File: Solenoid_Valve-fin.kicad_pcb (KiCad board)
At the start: 2 copper layers, 85.9 x 100 mm, 118 parts, among them IC1 Si8621AB-B-ISR, J1 Bus_mechaken_PCIexpress_x16_1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, J10 Conn_01x02, J11 Conn_01x02, J12 Conn_01x02, J13 Conn_01x02, J14 Conn_01x02, J15 Conn_01x02, J16 Conn_01x02, J17 Conn_01x02, J18 Conn_01x02, J19 Conn_01x02, J2 Conn_01x05, J20 Conn_01x02, J3 Conn_01x02, J4 Conn_01x02, J5 Conn_01x02, J6 Conn_01x02, J7 Conn_01x03, J8 Conn_01x02, J9 Conn_01x02, Q1 ULN2004D1013TR, Q2 ULN2004D1013TR, Q3 ULN2004D1013TR, U1 LDL1117S33R, U2 STM32F042K6Tx, U3 MCP2562-E-SN, U4 L7812, U5 LDL1117S33R

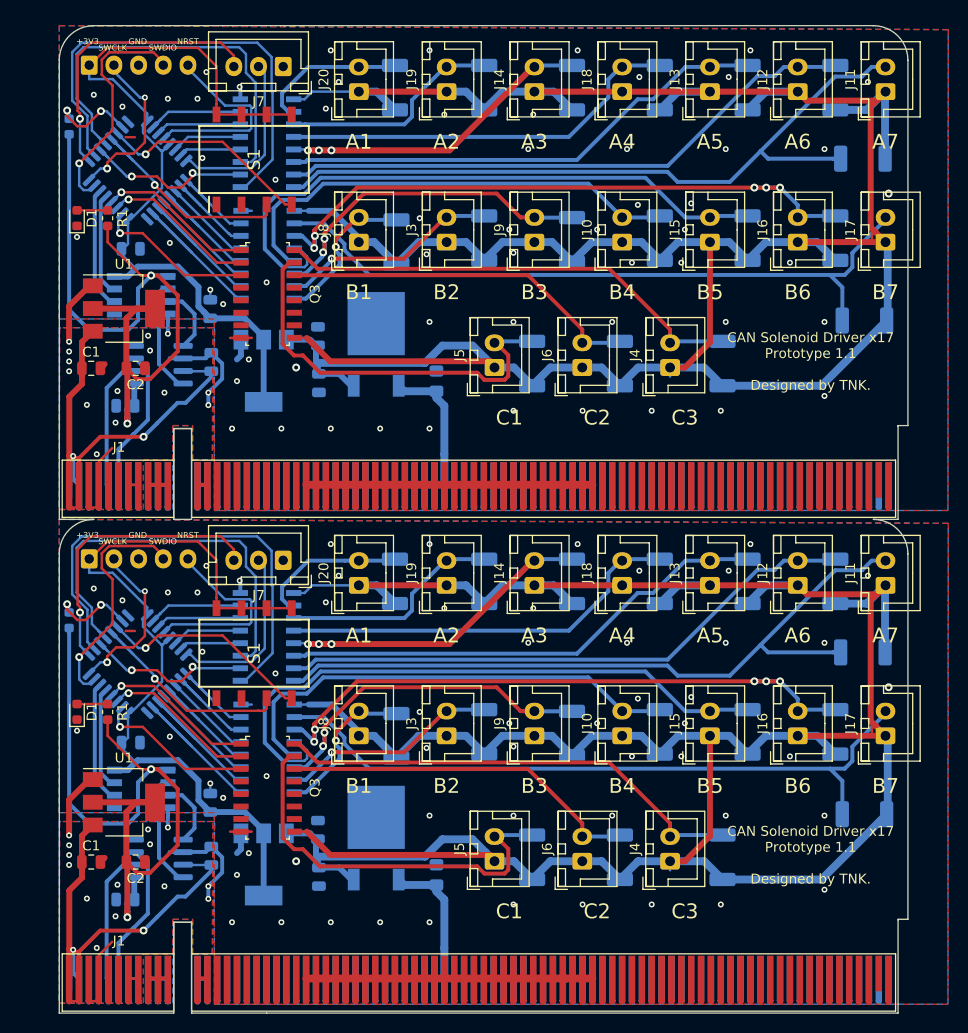
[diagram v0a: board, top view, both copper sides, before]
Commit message: Release
Prototype-1.3をリリース
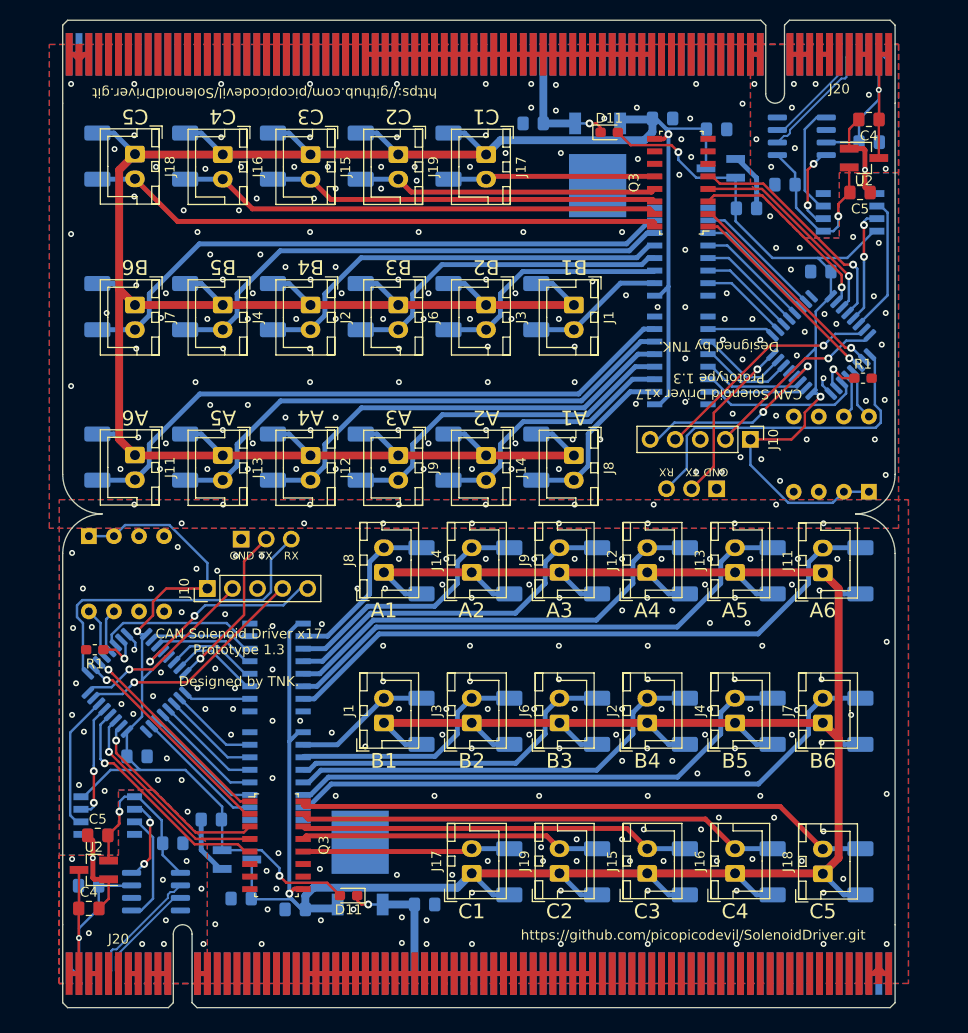
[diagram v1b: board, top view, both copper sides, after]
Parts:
- removed C10: 4.7uF, Capacitor_SMD:C_0805_2012Metric
- removed the D1 at (121.8, 49.5)
- removed the D1 at (121.8, 99.5)
- removed the D11 at (198.6, 36.3)
- removed D19: D, Diode_SMD:D_2010_5025Metric
- removed the R1 at (124.9, 49.5)
- removed the R1 at (124.9, 99.5)
- removed R2: 10K, Resistor_SMD:R_0603_1608Metric
- added C3: 0.1u, Capacitor_SMD:C_0805_2012Metric_Pad1.15x1.40mm_HandSolder, B.Cu at (181.1, 39.4)
- added D1: D, Diode_SMD:D_2010_5025Metric_Pad1.52x2.65mm_HandSolder, B.Cu at (168.3, 58.5)
- added D11: D_Schottky, Diode_SMD:D_0603_1608Metric_Pad1.05x0.95mm_HandSolder, F.Cu at (175.7, 40.8)
- added D11: D_Schottky, Diode_SMD:D_0603_1608Metric_Pad1.05x0.95mm_HandSolder, F.Cu at (149.3, 118.1)
- added D5: D, Diode_SMD:D_2010_5025Metric_Pad1.52x2.65mm_HandSolder, B.Cu at (150.5, 58.5)
- added R1: 10K, Resistor_SMD:R_0603_1608Metric_Pad1.05x0.95mm_HandSolder, F.Cu at (201.4, 65.7)
- C1: value 1.0uF -> 0.1u; footprint Capacitor_SMD:C_0805_2012Metric -> Capacitor_SMD:C_0805_2012Metric_Pad1.15x1.40mm_HandSolder; moved to B.Cu
- C1: renamed from C4; value 0.1uF -> 0.1u; footprint Capacitor_SMD:C_0805_2012Metric -> Capacitor_SMD:C_0805_2012Metric_Pad1.15x1.40mm_HandSolder
- C2: value 4.7uF -> 0.33u; footprint Capacitor_SMD:C_0805_2012Metric -> Capacitor_SMD:C_0805_2012Metric_Pad1.15x1.40mm_HandSolder; moved to B.Cu
- C2: renamed from C7; value 1uF -> 0.33u
- C3: renamed from C8; value 4.7uF -> 0.1u; footprint Capacitor_SMD:C_0805_2012Metric -> Capacitor_SMD:C_0805_2012Metric_Pad1.15x1.40mm_HandSolder
- C4: value 0.1uF -> 1.0u; footprint Capacitor_SMD:C_0805_2012Metric -> Capacitor_SMD:C_0805_2012Metric_Pad1.15x1.40mm_HandSolder; moved to F.Cu
- C4: renamed from C1; value 1.0uF -> 1.0u; footprint Capacitor_SMD:C_0805_2012Metric -> Capacitor_SMD:C_0805_2012Metric_Pad1.15x1.40mm_HandSolder
- C5: value 0.1uF -> 2.2u; footprint Capacitor_SMD:C_0805_2012Metric -> Capacitor_SMD:C_0805_2012Metric_Pad1.15x1.40mm_HandSolder; moved to F.Cu
- C5: renamed from C2; value 4.7uF -> 2.2u; footprint Capacitor_SMD:C_0805_2012Metric -> Capacitor_SMD:C_0805_2012Metric_Pad1.15x1.40mm_HandSolder
- C6 (x2): value 0.1uF -> 0.1u; footprint Capacitor_SMD:C_0805_2012Metric -> Capacitor_SMD:C_0805_2012Metric_Pad1.15x1.40mm_HandSolder
- C7: value 1uF -> 1.0u
- C7: renamed from C9; value 1.0uF -> 1.0u; footprint Capacitor_SMD:C_0805_2012Metric -> Capacitor_SMD:C_0805_2012Metric_Pad1.15x1.40mm_HandSolder
- C8: value 4.7uF -> 4.7u; footprint Capacitor_SMD:C_0805_2012Metric -> Capacitor_SMD:C_0805_2012Metric_Pad1.15x1.40mm_HandSolder
- C8: renamed from C10; value 4.7uF -> 4.7u; footprint Capacitor_SMD:C_0805_2012Metric -> Capacitor_SMD:C_0805_2012Metric_Pad1.15x1.40mm_HandSolder
- C9: value 1.0uF -> 0.1u; footprint Capacitor_SMD:C_0805_2012Metric -> Capacitor_SMD:C_0805_2012Metric_Pad1.15x1.40mm_HandSolder
- C9: renamed from C5; value 0.1uF -> 0.1u; footprint Capacitor_SMD:C_0805_2012Metric -> Capacitor_SMD:C_0805_2012Metric_Pad1.15x1.40mm_HandSolder
- D1: renamed from D6; footprint Diode_SMD:D_2010_5025Metric -> Diode_SMD:D_2010_5025Metric_Pad1.52x2.65mm_HandSolder
- D10, D12 (x2), D13, D14, D15, D16, D17, D18, D2, D3, D4, D6, D7, D8, D9: footprint Diode_SMD:D_2010_5025Metric -> Diode_SMD:D_2010_5025Metric_Pad1.52x2.65mm_HandSolder
- D10: renamed from D17; footprint Diode_SMD:D_2010_5025Metric -> Diode_SMD:D_2010_5025Metric_Pad1.52x2.65mm_HandSolder
- D13: renamed from D18; footprint Diode_SMD:D_2010_5025Metric -> Diode_SMD:D_2010_5025Metric_Pad1.52x2.65mm_HandSolder
- D14: renamed from D2; footprint Diode_SMD:D_2010_5025Metric -> Diode_SMD:D_2010_5025Metric_Pad1.52x2.65mm_HandSolder
- D15: renamed from D16; footprint Diode_SMD:D_2010_5025Metric -> Diode_SMD:D_2010_5025Metric_Pad1.52x2.65mm_HandSolder
- D16: renamed from D3; footprint Diode_SMD:D_2010_5025Metric -> Diode_SMD:D_2010_5025Metric_Pad1.52x2.65mm_HandSolder
- D17: renamed from D10; footprint Diode_SMD:D_2010_5025Metric -> Diode_SMD:D_2010_5025Metric_Pad1.52x2.65mm_HandSolder
- D18: renamed from D4; footprint Diode_SMD:D_2010_5025Metric -> Diode_SMD:D_2010_5025Metric_Pad1.52x2.65mm_HandSolder
- D2: renamed from D9; footprint Diode_SMD:D_2010_5025Metric -> Diode_SMD:D_2010_5025Metric_Pad1.52x2.65mm_HandSolder
- D3: renamed from D7; footprint Diode_SMD:D_2010_5025Metric -> Diode_SMD:D_2010_5025Metric_Pad1.52x2.65mm_HandSolder
- D4: renamed from D14; footprint Diode_SMD:D_2010_5025Metric -> Diode_SMD:D_2010_5025Metric_Pad1.52x2.65mm_HandSolder
- D5: renamed from D8; footprint Diode_SMD:D_2010_5025Metric -> Diode_SMD:D_2010_5025Metric_Pad1.52x2.65mm_HandSolder
- D6: renamed from D15; footprint Diode_SMD:D_2010_5025Metric -> Diode_SMD:D_2010_5025Metric_Pad1.52x2.65mm_HandSolder
- D7: renamed from D19; footprint Diode_SMD:D_2010_5025Metric -> Diode_SMD:D_2010_5025Metric_Pad1.52x2.65mm_HandSolder
- D8: renamed from D13; footprint Diode_SMD:D_2010_5025Metric -> Diode_SMD:D_2010_5025Metric_Pad1.52x2.65mm_HandSolder
- D9: renamed from D11; footprint Diode_SMD:D_2010_5025Metric -> Diode_SMD:D_2010_5025Metric_Pad1.52x2.65mm_HandSolder
- J1: value Bus_mechaken_PCIexpress_x16_164_Position -> Conn_01x02; footprint PCIe:BUS_mechaken_PCIexpress_x16_164_Position -> Connector_JST:JST_XH_B2B-XH-A_1x02_P2.50mm_Vertical
- J10: value Conn_01x02 -> Conn_01x05; footprint Connector_JST:JST_XH_B2B-XH-A_1x02_P2.50mm_Vertical -> Connector_PinHeader_2.54mm:PinHeader_1x05_P2.54mm_Vertical
- J10: renamed from J2; footprint Connector_JST:JST_XH_B5B-XH-A_1x05_P2.50mm_Vertical -> Connector_PinHeader_2.54mm:PinHeader_1x05_P2.54mm_Vertical; moved to F.Cu
- J2: value Conn_01x05 -> Conn_01x02; footprint Connector_JST:JST_XH_B5B-XH-A_1x05_P2.50mm_Vertical -> Connector_JST:JST_XH_B2B-XH-A_1x02_P2.50mm_Vertical; moved to F.Cu
- J20: value Conn_01x02 -> Bus_mechaken_PCIexpress_x16_164_Position; footprint Connector_JST:JST_XH_B2B-XH-A_1x02_P2.50mm_Vertical -> PCIe:BUS_mechaken_PCIexpress_x16
- J20: renamed from J1; footprint PCIe:BUS_mechaken_PCIexpress_x16_164_Position -> PCIe:BUS_mechaken_PCIexpress_x16
- J5: value Conn_01x02 -> Conn_01x03; footprint Connector_JST:JST_XH_B2B-XH-A_1x02_P2.50mm_Vertical -> Connector_PinHeader_2.54mm:PinHeader_1x03_P2.54mm_Vertical; moved to B.Cu
- J5: renamed from J7; footprint Connector_JST:JST_XH_B3B-XH-A_1x03_P2.50mm_Vertical -> Connector_PinHeader_2.54mm:PinHeader_1x03_P2.54mm_Vertical; moved to B.Cu
- J7: value Conn_01x03 -> Conn_01x02; footprint Connector_JST:JST_XH_B3B-XH-A_1x03_P2.50mm_Vertical -> Connector_JST:JST_XH_B2B-XH-A_1x02_P2.50mm_Vertical
- R1: renamed from R2; footprint Resistor_SMD:R_0603_1608Metric -> Resistor_SMD:R_0603_1608Metric_Pad1.05x0.95mm_HandSolder; moved to F.Cu
- S1 (x2): footprint SamacSys_Parts:SOP254P980X370-8N -> Package_DIP:DIP-8_W7.62mm; moved to B.Cu
- U1: value LDL1117S33R -> NJM7812; footprint Package_TO_SOT_SMD:SOT-223-3_TabPin2 -> Package_TO_SOT_SMD:TO-252-2; moved to B.Cu
- U1: renamed from U4; value L7812 -> NJM7812
- U2: value STM32F042K6Tx -> AP2210N-3.3TRG1; footprint Package_QFP:LQFP-32_7x7mm_P0.8mm -> Package_TO_SOT_SMD:SOT-23_Handsoldering; moved to F.Cu
- U2: renamed from U1; value LDL1117S33R -> AP2210N-3.3TRG1; footprint Package_TO_SOT_SMD:SOT-223-3_TabPin2 -> Package_TO_SOT_SMD:SOT-23_Handsoldering
- U3: value MCP2562-E-SN -> STM32F042K6Tx; footprint Package_SO:SOIC-8_3.9x4.9mm_P1.27mm -> Package_QFP:LQFP-32_7x7mm_P0.8mm
- U4: value L7812 -> AP2210N-3.3TRG1; footprint Package_TO_SOT_SMD:TO-252-2 -> Package_TO_SOT_SMD:SOT-23_Handsoldering
- U4: renamed from U5; value LDL1117S33R -> AP2210N-3.3TRG1; footprint Package_TO_SOT_SMD:SOT-223-3_TabPin2 -> Package_TO_SOT_SMD:SOT-23_Handsoldering
- U5: value LDL1117S33R -> MCP2562-E-SN; footprint Package_TO_SOT_SMD:SOT-223-3_TabPin2 -> Package_SO:SOIC-8_3.9x4.9mm_P1.27mm
- moved J11 84.5 mm to (127.7, 73.5), turned to 270 degrees
- moved C5 77.5 mm to (201.1, 46.9), turned to 180 degrees
- moved C4 75.9 mm to (202.0, 39.5)
- moved C1 74.5 mm to (197.1, 54.9)
- moved U2 73.6 mm to (201.5, 43.4), turned to 0 degrees
- moved IC1 72.3 mm to (200.1, 48.9), turned to 0 degrees
- moved S1 70.8 mm to (202.0, 77.2)
- moved C6 70.2 mm to (202.0, 41.8), turned to 180 degrees
- moved D12 68.1 mm to (132.8, 73.7), turned to 270 degrees
- moved U3 67.1 mm to (197.2, 62.3), turned to 45 degrees
- moved D10 67.0 mm to (141.6, 73.7), turned to 270 degrees
- moved D15 66.4 mm to (132.8, 43.2), turned to 270 degrees
- moved J12 61.6 mm to (145.4, 73.5), turned to 270 degrees
- moved J13 61.6 mm to (136.6, 73.5), turned to 270 degrees
- moved D9 61.1 mm to (123.9, 73.7), turned to 270 degrees
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- renumbered J8 to J1, J12 to J11, J18 to J12, J19 to J14, J4 to J15, J17 to J16, J5 to J17, J11 to J18, J6 to J19, J10 to J2, J15 to J4, J9 to J6, J16 to J7, J20 to J8, J14 to J9, U2 to U3, U3 to U5
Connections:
- C1 pad 1: +5V -> GNDPWR
- C1 pad 2: GND -> 3.3V
- C2 pad 1: GND -> VCC
- C2 pad 2: +3V3 -> GNDPWR
- C4 pad 1: GNDPWR -> +5V
- C4 pad 2: 3.3V -> GND
- C7 pad 1: VCC -> +12V
- C8 pad 1: +12V -> 3.3V
- C9 pad 1: +12V -> GND
- C9 pad 2: GNDPWR -> +3V3
- D1 pad 2: Solenoid_A1 -> Solenoid_B1
- D10 pad 2: Solenoid_B1 -> Solenoid_A4
- D10 pad 2: Solenoid_B5 -> Solenoid_A4
- D12 pad 2: Solenoid_B3 -> Solenoid_A5 (x2)
- D13 pad 2: Solenoid_B4 -> Solenoid_A2
- D13 pad 2: Solenoid_B6 -> Solenoid_A2
- D14 pad 2: Solenoid_A5 -> Solenoid_C3
- D14 pad 2: Solenoid_C1 -> Solenoid_C3
- D15 pad 2: Solenoid_A6 -> Solenoid_C4
- D15 pad 2: Solenoid_A7 -> Solenoid_C4
- D16 pad 2: Solenoid_A7 -> Solenoid_C1
- D16 pad 2: Solenoid_C2 -> Solenoid_C1
- D17 pad 2: Solenoid_B5 -> Solenoid_C5
- D17 pad 2: Solenoid_B1 -> Solenoid_C5
- D18 pad 2: Solenoid_B6 -> Solenoid_C2
- D18 pad 2: Solenoid_C3 -> Solenoid_C2
- D2 pad 2: Solenoid_C1 -> Solenoid_B4
- D2 pad 2: Solenoid_A4 -> Solenoid_B4
- D3 pad 2: Solenoid_C2 -> Solenoid_B2
- D3 pad 2: Solenoid_A2 -> Solenoid_B2
- D4 pad 2: Solenoid_C3 -> Solenoid_B5
- D4 pad 2: Solenoid_A5 -> Solenoid_B5
- D5 pad 2: Solenoid_A3 -> Solenoid_B3
- D6 pad 2: Solenoid_A1 -> Solenoid_B6
- D6 pad 2: Solenoid_A6 -> Solenoid_B6
- D7 pad 2: Solenoid_A2 -> Solenoid_A1
- D7 pad 2: Solenoid_B7 -> Solenoid_A1
- D8 pad 2: Solenoid_B4 -> Solenoid_A3
- D9 pad 2: Solenoid_A4 -> Solenoid_A6
- D9 pad 2: Solenoid_B2 -> Solenoid_A6
- J1 pad 2: Solenoid_A1 -> Solenoid_B1
- J10 pad 1: +12V -> 3.3V
- J10 pad 2: Solenoid_A4 -> /SWCLK
- J11 pad 2: Solenoid_B1 -> Solenoid_A6
- J11 pad 2: Solenoid_B2 -> Solenoid_A6
- J12 pad 2: Solenoid_B2 -> Solenoid_A4
- J12 pad 2: Solenoid_B5 -> Solenoid_A4
- J13 pad 2: Solenoid_B3 -> Solenoid_A5 (x2)
- J14 pad 2: Solenoid_B4 -> Solenoid_A2
- J14 pad 2: Solenoid_B6 -> Solenoid_A2
- J15 pad 2: Solenoid_A5 -> Solenoid_C3
- J15 pad 2: Solenoid_C1 -> Solenoid_C3
- J16 pad 2: Solenoid_A6 -> Solenoid_C4
- J16 pad 2: Solenoid_A7 -> Solenoid_C4
- J17 pad 2: Solenoid_A7 -> Solenoid_C1
- J17 pad 2: Solenoid_C2 -> Solenoid_C1
- J18 pad 2: Solenoid_B5 -> Solenoid_C5
- J18 pad 2: Solenoid_B1 -> Solenoid_C5
- J19 pad 2: Solenoid_B6 -> Solenoid_C2
- J19 pad 2: Solenoid_C3 -> Solenoid_C2
- J2 pad 1: 3.3V -> +12V
- J2 pad 2: /SWCLK -> Solenoid_B4
- J2 pad 2: Solenoid_A4 -> Solenoid_B4
- J20 pad A5: Net-(J1-PadA5) -> Net-(J20-PadA5)
- J20 pad A6: Net-(J1-PadA6) -> Net-(J20-PadA6)
- J20 pad A7: Net-(J1-PadA7) -> Net-(J20-PadA7)
- J20 pad B3: Net-(J1-PadB3) -> Net-(J20-PadB3)
- J20 pad B4: Net-(J1-PadB4) -> Net-(J20-PadB4)
- J20 pad B5: Net-(J1-PadB5) -> Net-(J20-PadB5)
- J20 pad B6: Net-(J1-PadB6) -> Net-(J20-PadB6)
- J20 pad B7: Net-(J1-PadB7) -> Net-(J20-PadB7)
- J20 pad B9: Net-(J1-PadB9) -> Net-(J20-PadB9)
- J3 pad 2: Solenoid_A2 -> Solenoid_B2 (x2)
- J4 pad 2: Solenoid_C1 -> Solenoid_B5
- J4 pad 2: Solenoid_A5 -> Solenoid_B5
- J5 pad 1: +12V -> GNDPWR
- J5 pad 2: Solenoid_C2 -> VCP_TX
- J6 pad 2: Solenoid_C3 -> Solenoid_B3
- J6 pad 2: Solenoid_A3 -> Solenoid_B3
- J7 pad 1: GNDPWR -> +12V
- J7 pad 2: VCP_TX -> Solenoid_B6
- J7 pad 2: Solenoid_A6 -> Solenoid_B6
- J8 pad 2: Solenoid_B7 -> Solenoid_A1
- J9 pad 2: Solenoid_B4 -> Solenoid_A3
- Q1 pad 1: IC_A1 -> Net-(Q1-Pad1) (x2)
- Q1 pad 10: Solenoid_A7 -> Solenoid_A1 (x2)
- Q1 pad 11: Solenoid_A6 -> Solenoid_A2 (x2)
- Q1 pad 12: Solenoid_A5 -> Solenoid_A3 (x2)
- Q1 pad 14: Solenoid_A3 -> Solenoid_A5 (x2)
- Q1 pad 15: Solenoid_A2 -> Solenoid_A6 (x2)
- Q1 pad 16: Solenoid_A1 -> Net-(Q1-Pad16) (x2)
- Q1 pad 2: IC_A2 -> IC_A6 (x2)
- Q1 pad 3: IC_A3 -> IC_A5 (x2)
- Q1 pad 5: IC_A5 -> IC_A3 (x2)
- Q1 pad 6: IC_A6 -> IC_A2 (x2)
- Q1 pad 7: IC_A7 -> IC_A1 (x2)
- Q2 pad 1: IC_B1 -> Net-(Q2-Pad1) (x2)
- Q2 pad 10: Solenoid_B7 -> Solenoid_B1 (x2)
- Q2 pad 11: Solenoid_B6 -> Solenoid_B2 (x2)
- Q2 pad 12: Solenoid_B5 -> Solenoid_B3 (x2)
- Q2 pad 14: Solenoid_B3 -> Solenoid_B5 (x2)
- Q2 pad 15: Solenoid_B2 -> Solenoid_B6 (x2)
- Q2 pad 16: Solenoid_B1 -> Net-(Q2-Pad16) (x2)
- Q2 pad 2: IC_B2 -> IC_B6 (x2)
- Q2 pad 3: IC_B3 -> IC_B5 (x2)
- Q2 pad 5: IC_B5 -> IC_B3 (x2)
- Q2 pad 6: IC_B6 -> IC_B2 (x2)
- Q2 pad 7: IC_B7 -> IC_B1 (x2)
- Q3 pad 1: IC_C1 -> IC_C5 (x2)
- Q3 pad 10: (no net) -> Net-(Q3-Pad10) (x2)
- Q3 pad 11: (no net) -> Net-(Q3-Pad11) (x2)
- Q3 pad 12: (no net) -> Solenoid_C1 (x2)
- Q3 pad 13: (no net) -> Solenoid_C2 (x2)
- Q3 pad 15: Solenoid_C2 -> Solenoid_C4 (x2)
- Q3 pad 16: Solenoid_C1 -> Solenoid_C5 (x2)
- Q3 pad 2: IC_C2 -> IC_C4 (x2)
- Q3 pad 4: (no net) -> IC_C2 (x2)
- Q3 pad 5: (no net) -> IC_C1 (x2)
- Q3 pad 6: (no net) -> Net-(Q3-Pad6) (x2)
- Q3 pad 7: (no net) -> Net-(Q3-Pad7) (x2)
- R1 pad 2: +3V3 -> GNDPWR
- S1 pad 1: (no net) -> 3.3V (x2)
- S1 pad 2: (no net) -> 3.3V (x2)
- S1 pad 3: DIP_SW_1 -> Net-(S1-Pad3) (x2)
- S1 pad 4: DIP_SW_2 -> Net-(S1-Pad4) (x2)
- S1 pad 5: 3.3V -> Net-(S1-Pad5) (x2)
- S1 pad 6: 3.3V -> Net-(S1-Pad6) (x2)
- S1 pad 7: 3.3V -> DIP_SW_2 (x2)
- S1 pad 8: 3.3V -> DIP_SW_1 (x2)
- U1 pad 1: GND -> VCC
- U1 pad 2: +3V3 -> GNDPWR
- U1 pad 3: +5V -> +12V
- U2 pad 1: 3.3V -> GND
- U2 pad 2: IC_B7 -> +3V3
- U2 pad 3: IC_B6 -> +5V
- U3 pad 1: CAN_TXD -> 3.3V
- U3 pad 2: GND -> IC_A2
- U3 pad 3: +5V -> IC_A3
- U3 pad 4: CAN_RXD -> NRST
- U3 pad 5: +3V3 -> 3.3V
- U3 pad 6: CAN- -> IC_A4
- U3 pad 7: CAN+ -> IC_A5
- U3 pad 8: GND -> VCP_TX
- U3 pad 10: IC_A6 -> IC_B1
- U3 pad 11: IC_A5 -> IC_B2
- U3 pad 12: IC_A4 -> IC_B3
- U3 pad 13: IC_A3 -> IC_B4
- U3 pad 14: IC_A2 -> IC_B5
- U3 pad 15: IC_A1 -> IC_B6
- U3 pad 2: IC_B7 -> IC_A2
- U3 pad 26: IC_B1 -> IC_C4
- U3 pad 27: IC_B2 -> IC_C5
- U3 pad 28: IC_B3 -> DIP_SW_1
- U3 pad 29: DIP_SW_1 -> DIP_SW_2
- U3 pad 3: IC_B6 -> IC_A3
- U3 pad 30: DIP_SW_2 -> IC_A1
- U3 pad 6: IC_B5 -> IC_A4
- U3 pad 7: IC_B4 -> IC_A5
- U3 pad 9: IC_A7 -> IC_A6
- U4 pad 1: VCC -> GNDPWR
- U4 pad 2: GNDPWR -> 3.3V
- U5 pad 1: GNDPWR -> CAN_TXD
- U5 pad 2: 3.3V -> GND
- U5 pad 3: +12V -> +5V
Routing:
- net Solenoid_A7: track 141.4 -> 0.00 mm
- net +3V3: track 164.7 -> 36.4 mm, vias 4 -> 2
- net +12V: track 733.2 -> 610.2 mm, vias 0 -> 2
- net Solenoid_B1: track 148.5 -> 27.9 mm
- net Solenoid_C5: track 0.00 -> 117.3 mm
- net Solenoid_C4: track 0.00 -> 98.0 mm
- net Solenoid_B6: track 45.5 -> 124.6 mm
- net IC_B1: track 94.8 -> 18.1 mm
- net Solenoid_B2: track 118.9 -> 49.3 mm
- net +5V: track 117.1 -> 51.9 mm, vias 4 -> 2
- net IC_B3: track 83.3 -> 21.5 mm
- net Net-(J20-PadB9): track 0.00 -> 58.0 mm
- net Net-(J1-PadB9): track 58.0 -> 0.00 mm
- net Solenoid_C1: track 97.0 -> 41.2 mm
- net IC_C4: track 0.00 -> 44.3 mm, vias 0 -> 2
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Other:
- board size 85.9 x 100 mm -> 84.3 x 83.2 mm
- board text added: "3V3"
- board text added: "C4"
- board text added: "C5"
- board text added: "CAN Solenoid Driver x17 Prototype 1.3 Designed by TNK."
- board text added: "RX"
- board text added: "TX"
- board text added: "https://github.com/picopicodevil/SolenoidDriver.git"
- board text removed: "+3V3"
- board text removed: "A7"
- board text removed: "B7"
- board text removed: "CAN Solenoid Driver x17 Prototype 1.1 Designed by TNK."
- board text removed: "VCP_TX"
- board text removed: "VXP_TX"
